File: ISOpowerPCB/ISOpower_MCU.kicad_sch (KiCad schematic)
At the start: 5 parts

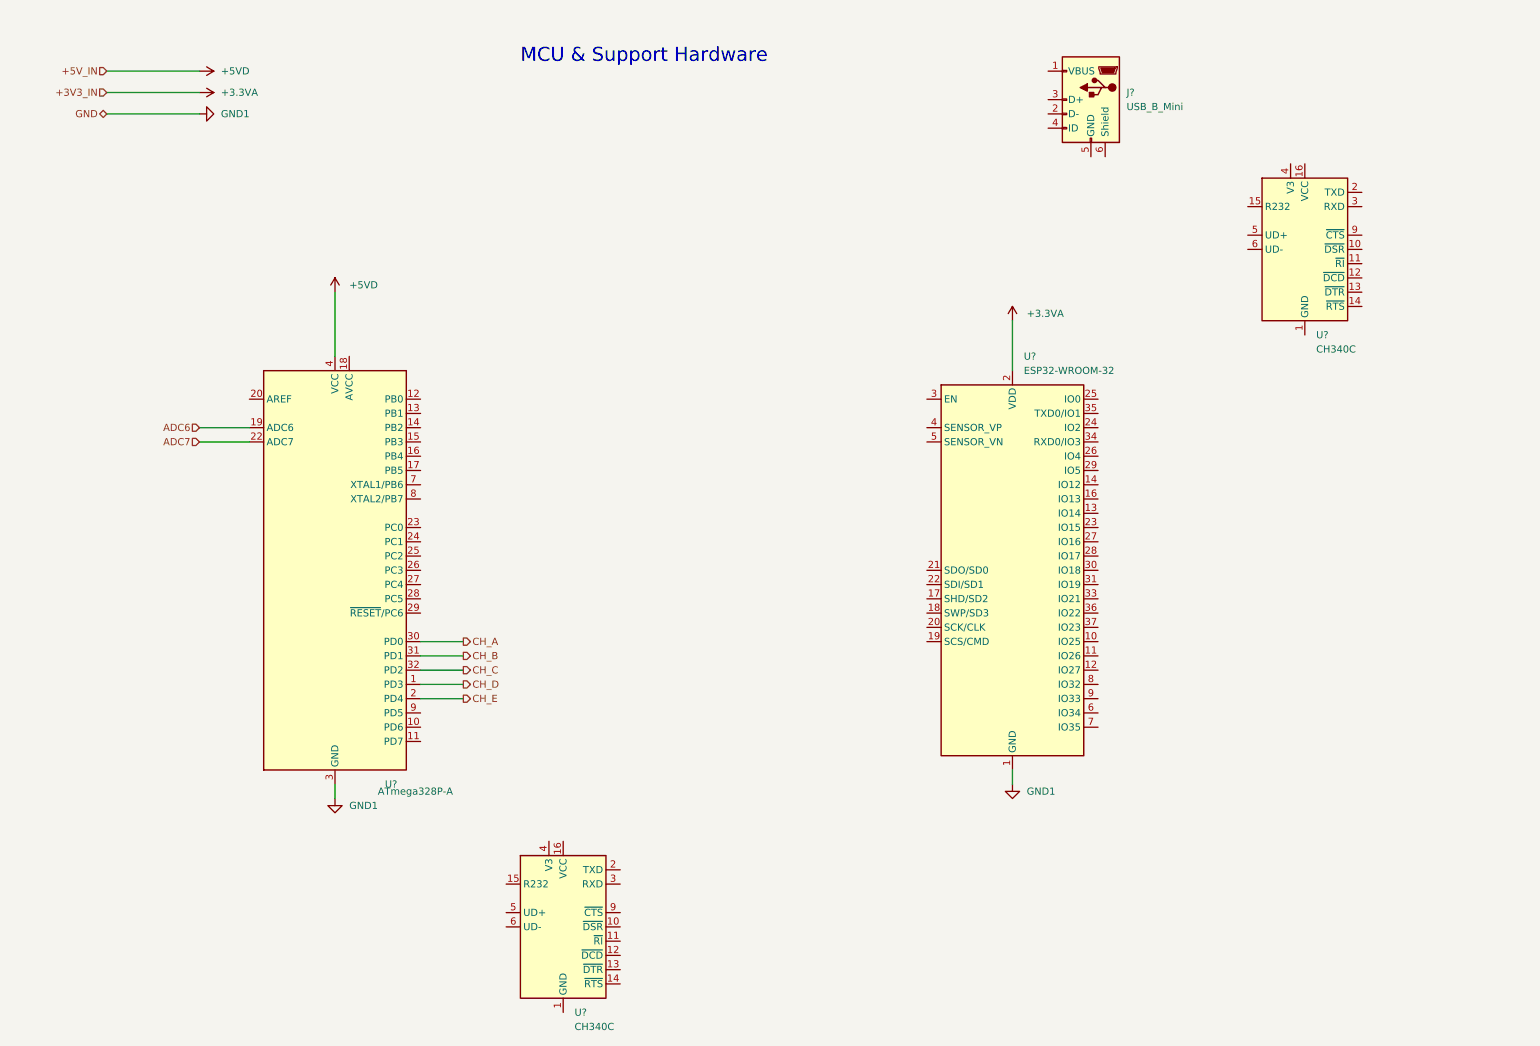
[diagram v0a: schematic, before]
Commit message: deleted old backups & added documentation
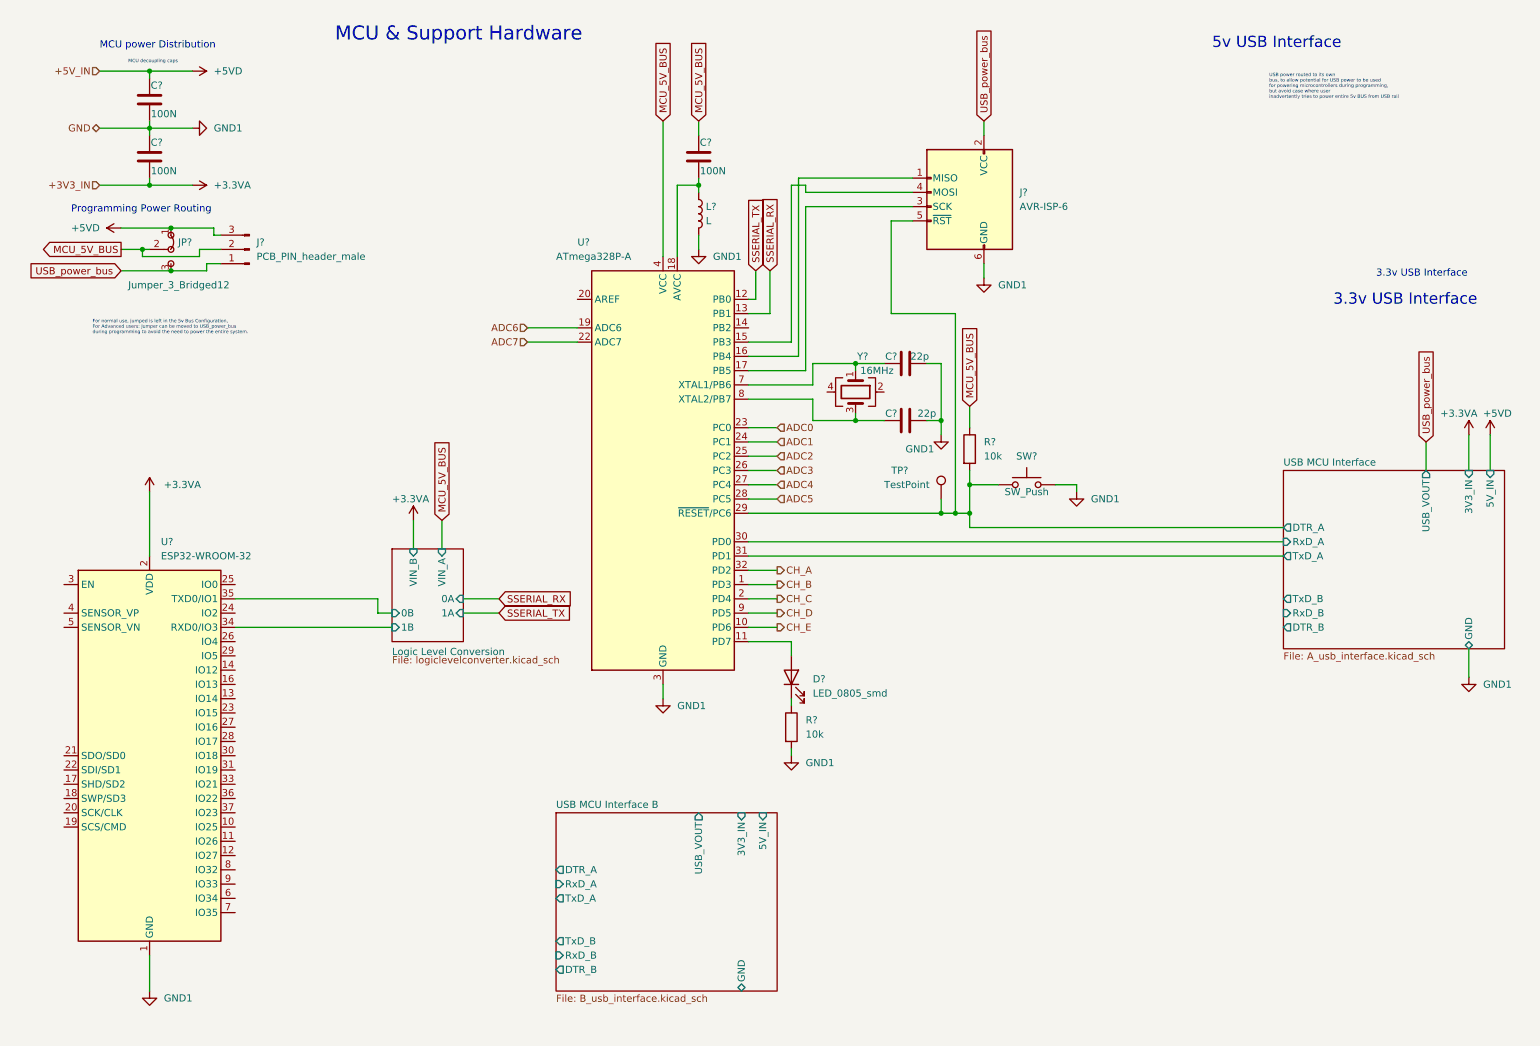
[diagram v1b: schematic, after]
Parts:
- removed J?: USB_B_Mini, symbol Connector:USB_B_Mini
- removed U? (x2): CH340C, Package_SO:SOIC-16_3.9x9.9mm_P1.27mm, symbol Interface_USB:CH340C
- added C? (x3): 100N, Capacitor_SMD:C_0805_2012Metric_Pad1.18x1.45mm_HandSolder, symbol 000_Capacitor_film_immo:cap_film_0805
- added C? (x2): 22p, Capacitor_SMD:C_0805_2012Metric_Pad1.18x1.45mm_HandSolder, symbol 000_Capacitor_film_immo:cap_film_0805
- added D?: LED_0805_smd, Diode_SMD:D_0805_2012Metric_Pad1.15x1.40mm_HandSolder, symbol 000_Diodes_Immo:LED_0805_smd
- added J?: PCB_PIN_header_male, symbol Connector:Conn_01x03_Male
- added J?: AVR-ISP-6, symbol Connector:AVR-ISP-6
- added JP?: Jumper_3_Bridged12, symbol 000_Connectors_Immo:Jumper_3_Bridged12
- added L?: L, symbol Device:L
- added R? (x2): 10k, Resistor_SMD:R_0805_2012Metric_Pad1.20x1.40mm_HandSolder, symbol 000_Resistors_Immo:Resistor_0805
- added SW?: SW_Push, symbol Switch:SW_Push
- added TP?: TestPoint, symbol Connector:TestPoint
- added Y?: 16MHz, symbol Device:Crystal_GND24
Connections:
- net +3.3VA: now also C?.2
- net +5VD: now also C?.1, J?.3 (Pin_3), JP?.1 (A); no longer U?.4 (VCC), U?.6 (VCC)
- net CH_A: now also U?.32 (PD2); no longer U?.30 (PD0)
- net CH_B: now also U?.1 (PD3); no longer U?.31 (PD1)
- net CH_C: now also U?.2 (PD4); no longer U?.32 (PD2)
- net CH_D: now also U?.9 (PD5); no longer U?.1 (PD3)
- net CH_E: now also U?.10 (PD6); no longer U?.2 (PD4)
- net GND1: now also C?.1, C?.2, C?.2, C?.2, J?.6 (GND), L?.2, R?.2, SW?.2
- net Logic Level Conversion/1B: now reaches U?.34 (RXD0/IO3)
- net Logic Level Conversion/0B: now reaches U?.35 (TXD0/IO1)
- net at U?.11 (PD7): now also D?.2 (A)
- net SSERIAL_TX: now reaches U?.12 (PB0)
- net SSERIAL_RX: now reaches U?.13 (PB1)
- net at U?.15 (PB3): now also J?.4 (MOSI)
- net at U?.16 (PB4): now also J?.1 (MISO)
- net at U?.17 (PB5): now also J?.3 (SCK)
- net at U?.18 (AVCC): now also C?.2, L?.1
- net ADC0: now reaches U?.23 (PC0)
- net ADC1: now reaches U?.24 (PC1)
- net ADC2: now reaches U?.25 (PC2)
- net ADC3: now reaches U?.26 (PC3)
- net ADC4: now reaches U?.27 (PC4)
- net ADC5: now reaches U?.28 (PC5)
- net USB MCU Interface/DTR_A: now reaches U?.29 (~{RESET}/PC6)
- net USB MCU Interface/DTR_A: now also J?.5 (~{RST}), R?.2, SW?.1, TP?.1
- net at U?.7 (XTAL1/PB6): now also C?.1, Y?.1
- net at U?.8 (XTAL2/PB7): now also C?.1, Y?.3
- new net: D?.1 (K), R?.1
- new net MCU_5V_BUS: C?.1, J?.2 (Pin_2), JP?.2 (C), R?.1, U?.4 (VCC), U?.6 (VCC)
- new net USB MCU Interface/RxD_A: U?.30 (PD0)
- new net USB MCU Interface/TxD_A: U?.31 (PD1)
- new net USB_power_bus: J?.1 (Pin_1), J?.2 (VCC), JP?.3 (B)
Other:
- added sheet Logic Level Conversion (logiclevelconverter.kicad_sch)
- added sheet USB MCU Interface (A_usb_interface.kicad_sch)
- added sheet USB MCU Interface B (B_usb_interface.kicad_sch)
- note added: "3.3v USB Interface"
- note added: "5v USB Interface"
- note added: "For normal use, jumped is left in the 5v Bus Configuration, For Advanced users: Jumper can be moved to USB_power_bus during programming to avoid the need to power the entire system."
- note added: "MCU decoupling caps"
- note added: "MCU power Distribution"
- note added: "Programming Power Routing"
- note added: "USB power routed to its own bus, to allow potential for USB power to be used for powering microcontrollers during programming, but avoid case where user inadvertently tries to power entire 5v BUS from USB rail"
- moved on the sheet: U?
